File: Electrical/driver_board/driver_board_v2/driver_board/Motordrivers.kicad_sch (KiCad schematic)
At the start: 30 parts, among them J4 Conn_01x04_Socket, J5 Conn_01x04_Socket, J6 Conn_01x04_Socket, J7 Conn_01x04_Socket, J8 Conn_01x04_Socket, J9 Conn_01x04_Socket

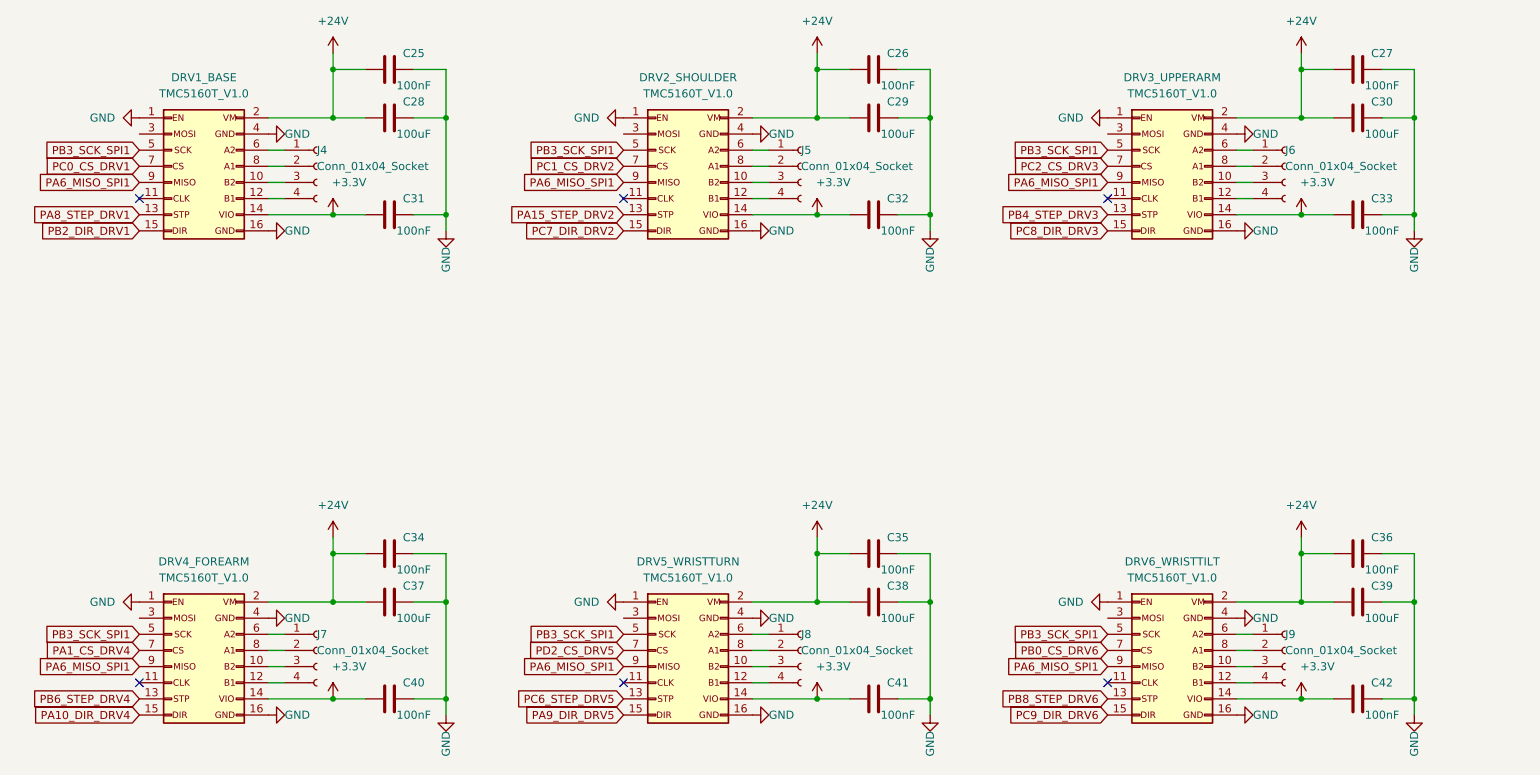
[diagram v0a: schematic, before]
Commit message: Finished TMC Labeling
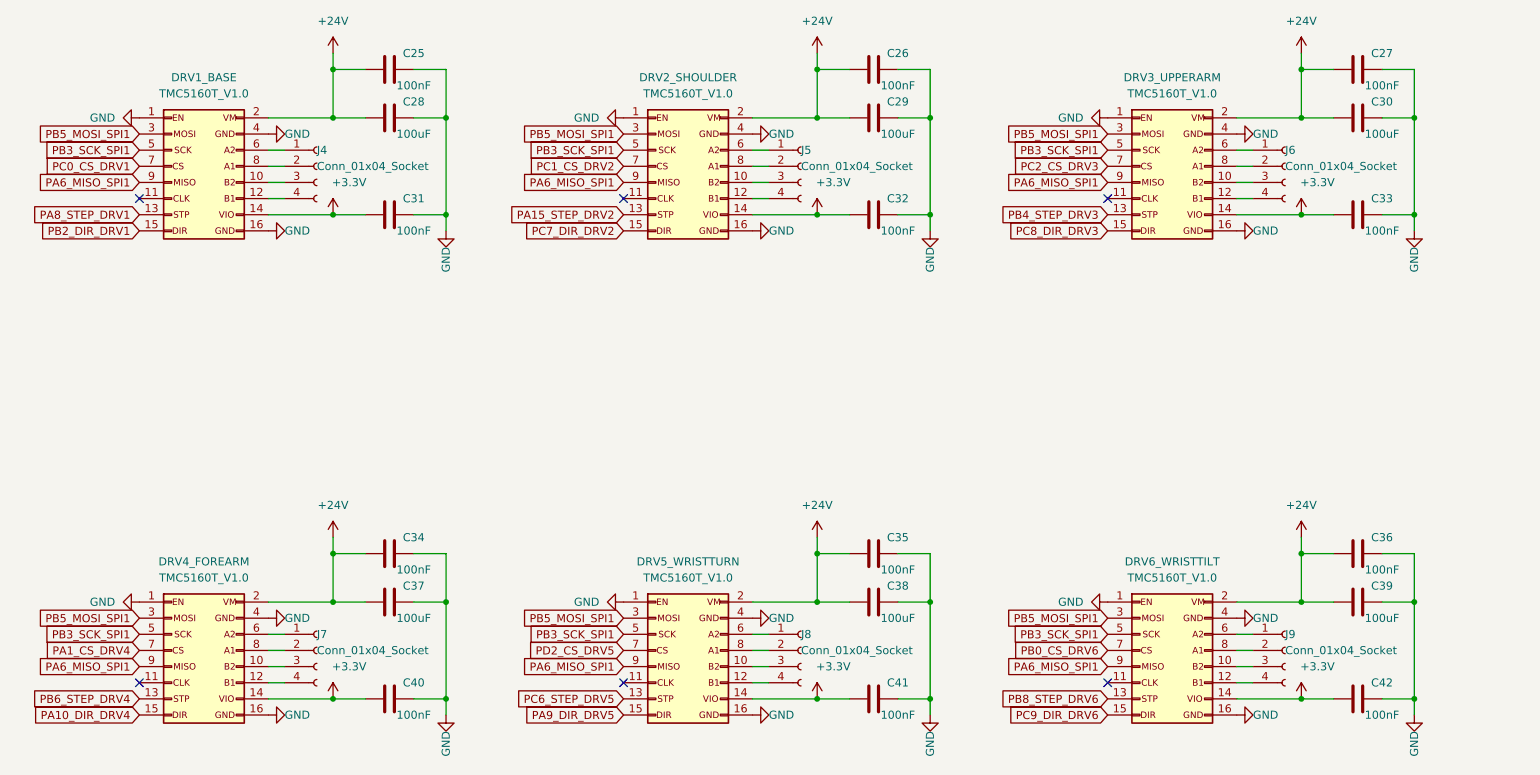
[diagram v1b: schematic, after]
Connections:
- net PB5_MOSI_SPI1: now reaches DRV2_SHOULDER.3 (Pin_3)
- net PB5_MOSI_SPI1: now also DRV1_BASE.3 (Pin_3), DRV3_UPPERARM.3 (Pin_3), DRV4_FOREARM.3 (Pin_3), DRV5_WRISTTURN.3 (Pin_3), DRV6_WRISTTILT.3 (Pin_3)
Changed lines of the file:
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@@
+		)
+	)
+	(global_label "PB5_MOSI_SPI1"
+		(shape input)
+		(at 40.64 121.92 180)
+		(fields_autoplaced yes)
+		(effects
+			(font
+				(size 1.27 1.27)
+			)
+			(justify right)
+		)
+		(property "Intersheetrefs" "${INTERSHEET_REFS}"
+			(at 23.0801 121.92 0)
+			(effects
+				(font
+					(size 1.27 1.27)
+				)
+				(justify right)
+				(hide yes)
+			)
 		)
 	)
@@
 		)
 	)
+	(global_label "PB5_MOSI_SPI1"
+		(shape input)
+		(at 193.04 45.72 180)
+		(fields_autoplaced yes)
+		(effects
+			(font
+				(size 1.27 1.27)
+			)
+			(justify right)
+		)
+		(property "Intersheetrefs" "${INTERSHEET_REFS}"
+			(at 175.4801 45.72 0)
+			(effects
+				(font
+					(size 1.27 1.27)
+				)
+				(justify right)
+				(hide yes)
+			)
+		)
+	)
 	(global_label "PB2_DIR_DRV1"
 		(shape input)
@@
 		)
 	)
+	(global_label "PB5_MOSI_SPI1"
+		(shape input)
+		(at 40.64 45.72 180)
+		(fields_autoplaced yes)
+		(effects
+			(font
+				(size 1.27 1.27)
+			)
+			(justify right)
+		)
+		(property "Intersheetrefs" "${INTERSHEET_REFS}"
+			(at 23.0801 45.72 0)
+			(effects
+				(font
+					(size 1.27 1.27)
+				)
+				(justify right)
+				(hide yes)
+			)
+		)
+	)
 	(global_label "PC0_CS_DRV1"
 		(shape input)
@@
 		)
 	)
+	(global_label "PB5_MOSI_SPI1"
+		(shape input)
+		(at 116.84 45.72 180)
+		(fields_autoplaced yes)
+		(effects
+			(font
+				(size 1.27 1.27)
+			)
+			(justify right)
+		)
+		(property "Intersheetrefs" "${INTERSHEET_REFS}"
+			(at 99.2801 45.72 0)
+			(effects
+				(font
+					(size 1.27 1.27)
+				)
+				(justify right)
+				(hide yes)
+			)
+		)
+	)
 	(global_label "PB8_STEP_DRV6"
 		(shape input)
@@
 		)
 	)
+	(global_label "PB5_MOSI_SPI1"
+		(shape input)
+		(at 193.04 121.92 180)
+		(fields_autoplaced yes)
+		(effects
+			(font
+				(size 1.27 1.27)
+			)
+			(justify right)
+		)
+		(property "Intersheetrefs" "${INTERSHEET_REFS}"
+			(at 175.4801 121.92 0)
+			(effects
+				(font
+					(size 1.27 1.27)
+				)
+				(justify right)
+				(hide yes)
+			)
+		)
+	)
 	(global_label "PC6_STEP_DRV5"
 		(shape input)
@@
 			(effects
 				(font
+					(size 1.27 1.27)
+				)
+				(justify right)
+				(hide yes)
+			)
+		)
+	)
+	(global_label "PB5_MOSI_SPI1"
+		(shape input)
+		(at 116.84 121.92 180)
+		(fields_autoplaced yes)
+		(effects
+			(font
+				(size 1.27 1.27)
+			)
+			(justify right)
+		)
+		(property "Intersheetrefs" "${INTERSHEET_REFS}"
+			(at 99.2801 121.92 0)
+			(effects
+				(font

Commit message: Added gnd plane
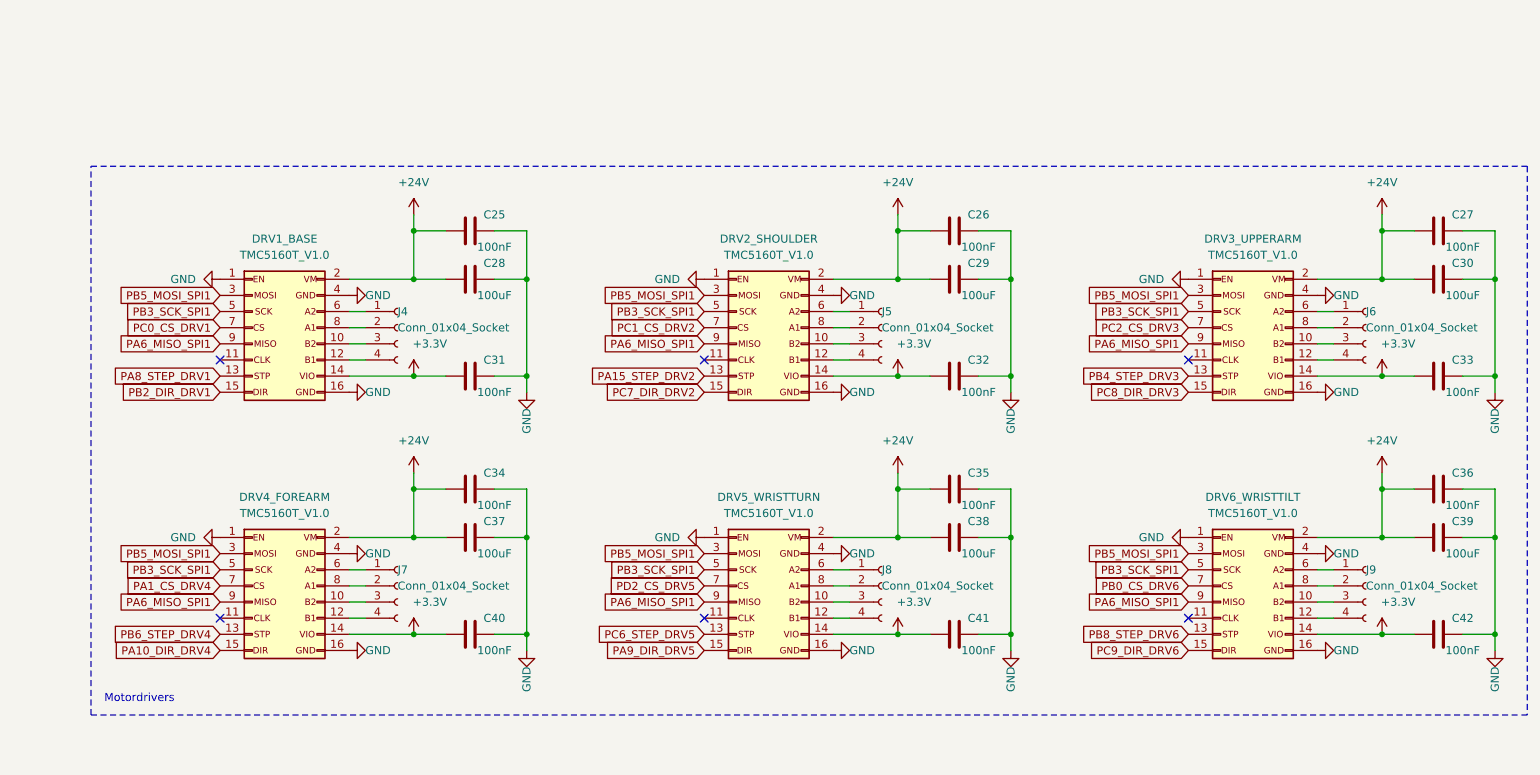
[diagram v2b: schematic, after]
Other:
- note added: "Motordrivers"
- moved on the sheet: C25, C26, C27, C28, C29, C30, C31, C32, C33, C34, C35, C36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
